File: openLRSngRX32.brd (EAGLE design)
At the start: 48.6 x 48.2 mm, 49 parts, among them IC1 STM32F10XCXT6, IC2 REG1117, U1 MPU-6000QFN-24

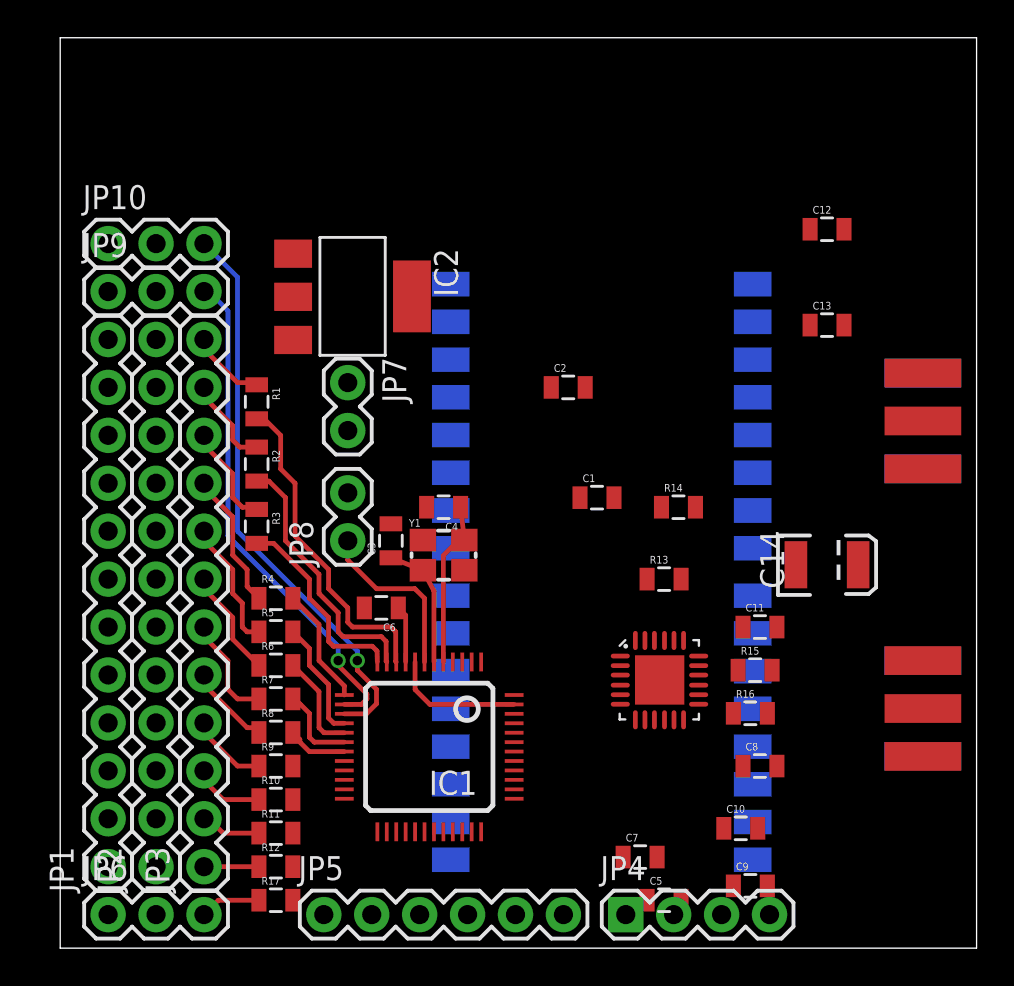
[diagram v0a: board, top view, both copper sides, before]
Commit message: updates
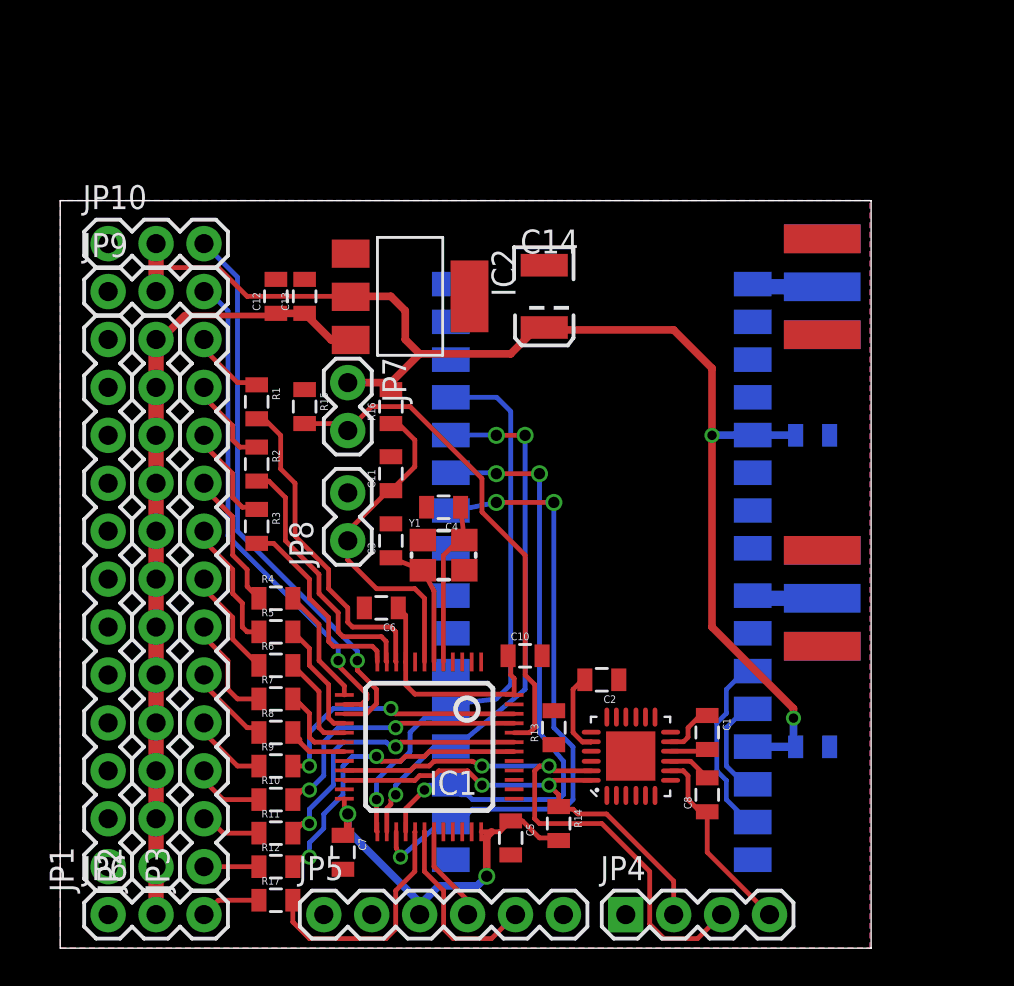
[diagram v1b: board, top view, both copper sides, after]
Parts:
- added C15: (no value), SparkFun-Capacitors:0805
- moved C12 29.4 mm to (11.4, 34.5), turned to 90 degrees
- moved C13 27.7 mm to (13.0, 34.5), turned to 90 degrees
- moved R15 27.7 mm to (13.0, 28.7), turned to 270 degrees
- moved R16 25.0 mm to (17.5, 28.7), turned to 90 degrees
- moved C11 21.2 mm to (17.5, 25.1), turned to 90 degrees
- moved C14 20.7 mm to (25.7, 34.5), turned to 270 degrees
- moved R14 17.9 mm to (26.4, 6.60), turned to 270 degrees
- moved C7 15.8 mm to (15.0, 5.08), turned to 270 degrees
- moved C2 15.6 mm to (28.7, 14.2), turned to 180 degrees
- moved C10 14.6 mm to (24.6, 15.5)
- moved C1 13.7 mm to (34.3, 11.4), turned to 270 degrees
- moved R13 9.80 mm to (26.2, 11.7), turned to 90 degrees
- moved J$2 8.89 mm to (40.4, 32.5), flipped to the bottom
- moved C5 8.77 mm to (23.9, 5.84), turned to 270 degrees
- moved C9 8.07 mm to (39.9, 10.7), flipped to the bottom, turned to 180 degrees
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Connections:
- net 3V3: now also C15.1
- net GND: now also C15.2
- net PWM10: now also IC1.45; no longer IC1.43
- net PWM11: now also IC1.43; no longer IC1.45
- net PWM12: now also IC1.42; no longer IC1.46
- net PWM9: now also IC1.46; no longer IC1.42
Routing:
- net 3V3: track 3.03 -> 116.4 mm, vias 0 -> 4
- net VCC: track 0.00 -> 42.0 mm
- net MISO: track 0.00 -> 33.7 mm, vias 0 -> 3
- net MOSI: track 0.00 -> 32.8 mm, vias 0 -> 3
- net SCL: track 0.00 -> 31.6 mm, vias 0 -> 2
- net NSS: track 0.00 -> 30.4 mm, vias 0 -> 1
- net SCK: track 0.00 -> 28.8 mm, vias 0 -> 3
- net BOOT0: track 0.00 -> 27.2 mm
- net SDA: track 0.00 -> 24.6 mm, vias 0 -> 2
- net PWM12: track 0.00 -> 16.3 mm, vias 0 -> 2
- net PWM11: track 0.00 -> 15.4 mm, vias 0 -> 2
- net PWM10: track 0.00 -> 14.4 mm, vias 0 -> 2
- net PWM9: track 0.00 -> 14.2 mm, vias 0 -> 2
- net PPM: track 0.00 -> 12.8 mm
- net TX: track 0.00 -> 10.1 mm
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- added copper zone on layer 1, net GND
- added copper zone on layer 16, net GND
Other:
- board size 48.6 x 48.2 mm -> 43 x 39.6 mm
